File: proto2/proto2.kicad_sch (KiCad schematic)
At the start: 9 parts, among them J13 Daughter Card, SW1 SW_DIP_x04

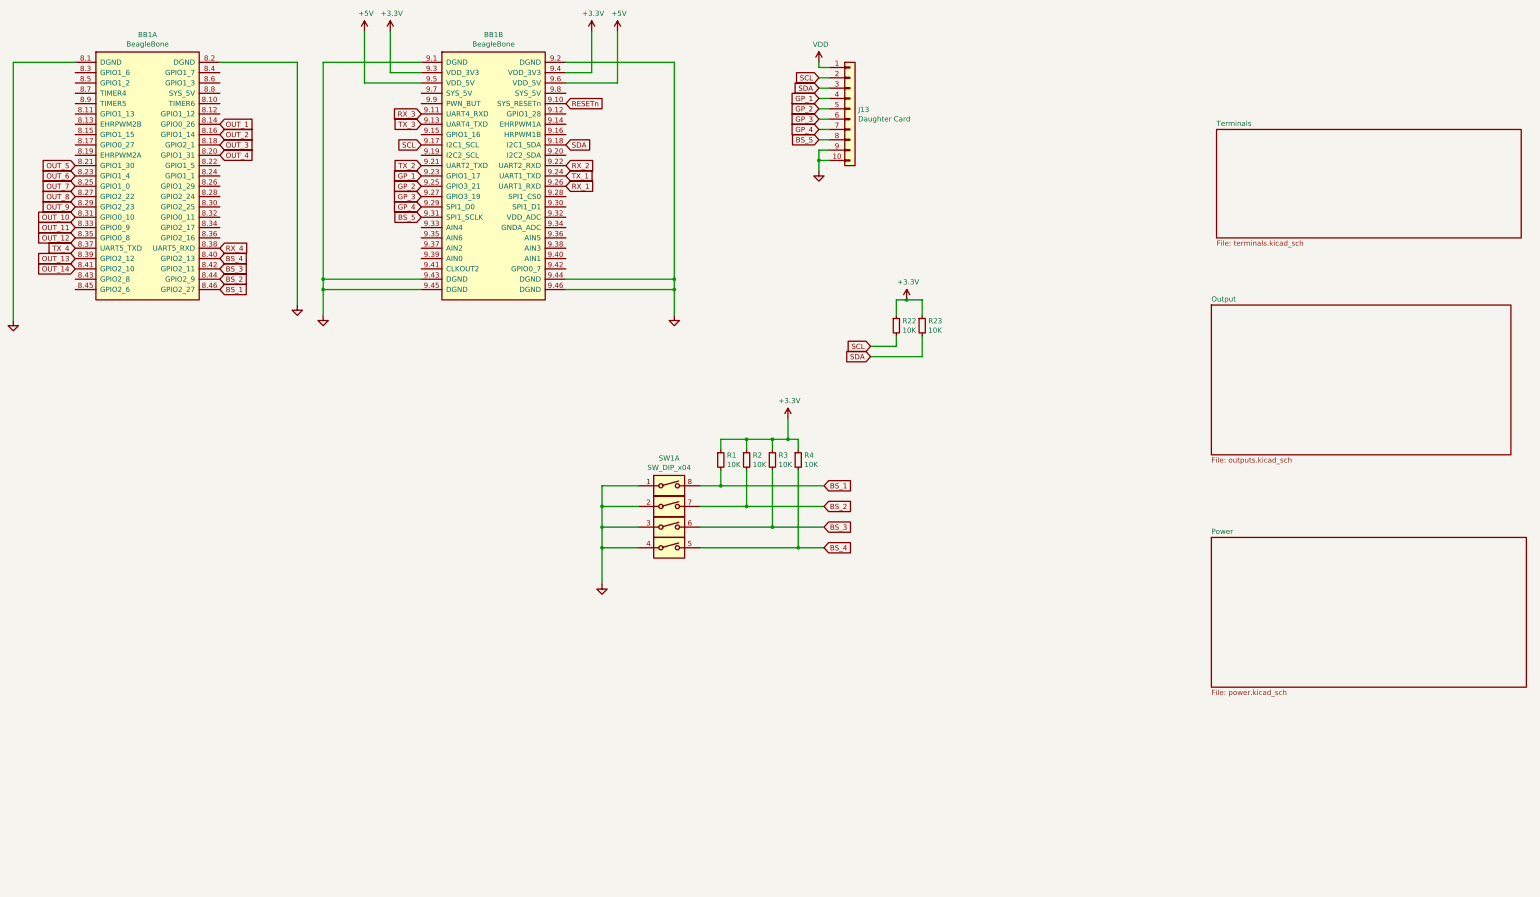
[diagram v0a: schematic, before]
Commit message: Working in suggestions from CFL review.
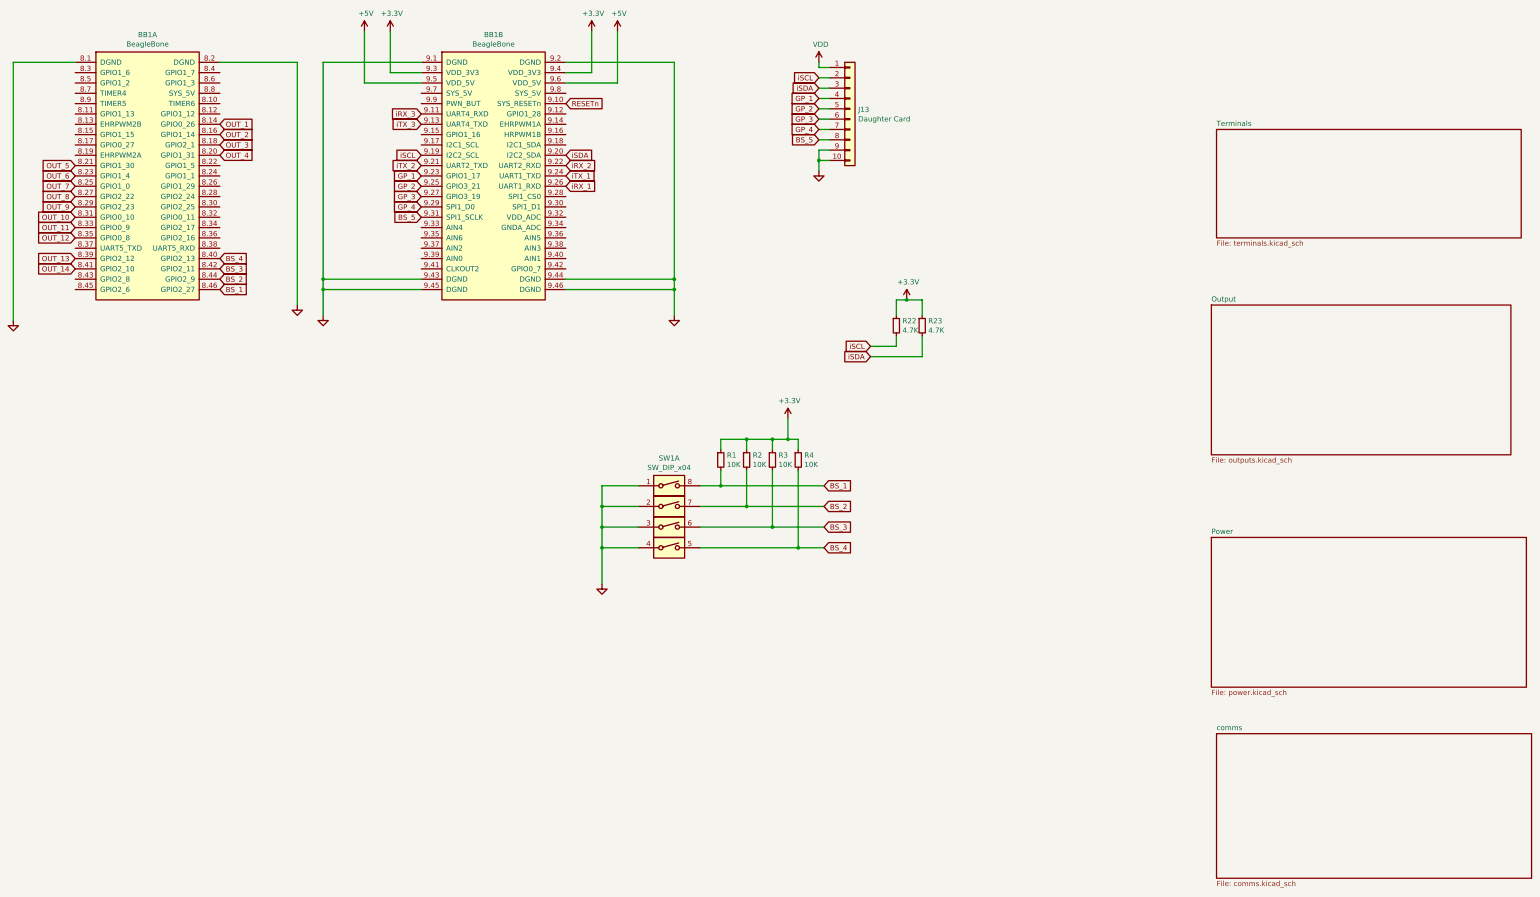
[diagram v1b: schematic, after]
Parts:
- R22, R23: value 10K -> 4.7K; LCSC C17414 -> C17673
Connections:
- net iSCL: now reaches BB1.9.19 (I2C2_SCL)
- net iSCL: now also J13.2 (Pin_2), R22.2
- net iSDA: now reaches BB1.9.20 (I2C2_SDA)
- net iSDA: now also J13.3 (Pin_3), R23.2
- net RX_1 renamed iRX_1
- net RX_2 renamed iRX_2
- net RX_3 renamed iRX_3
- net RX_4: no longer names the net of BB1.8.38 (UART5_RXD)
- removed net SCL: BB1.9.17 (I2C1_SCL), J13.2 (Pin_2), R22.2
- removed net SDA: BB1.9.18 (I2C1_SDA), J13.3 (Pin_3), R23.2
- net TX_1 renamed iTX_1
- net TX_2 renamed iTX_2
- net TX_3 renamed iTX_3
- net TX_4: no longer names the net of BB1.8.37 (UART5_TXD)
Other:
- added sheet comms (comms.kicad_sch)
